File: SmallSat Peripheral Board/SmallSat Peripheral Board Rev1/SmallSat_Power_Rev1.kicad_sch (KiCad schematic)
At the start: 23 parts

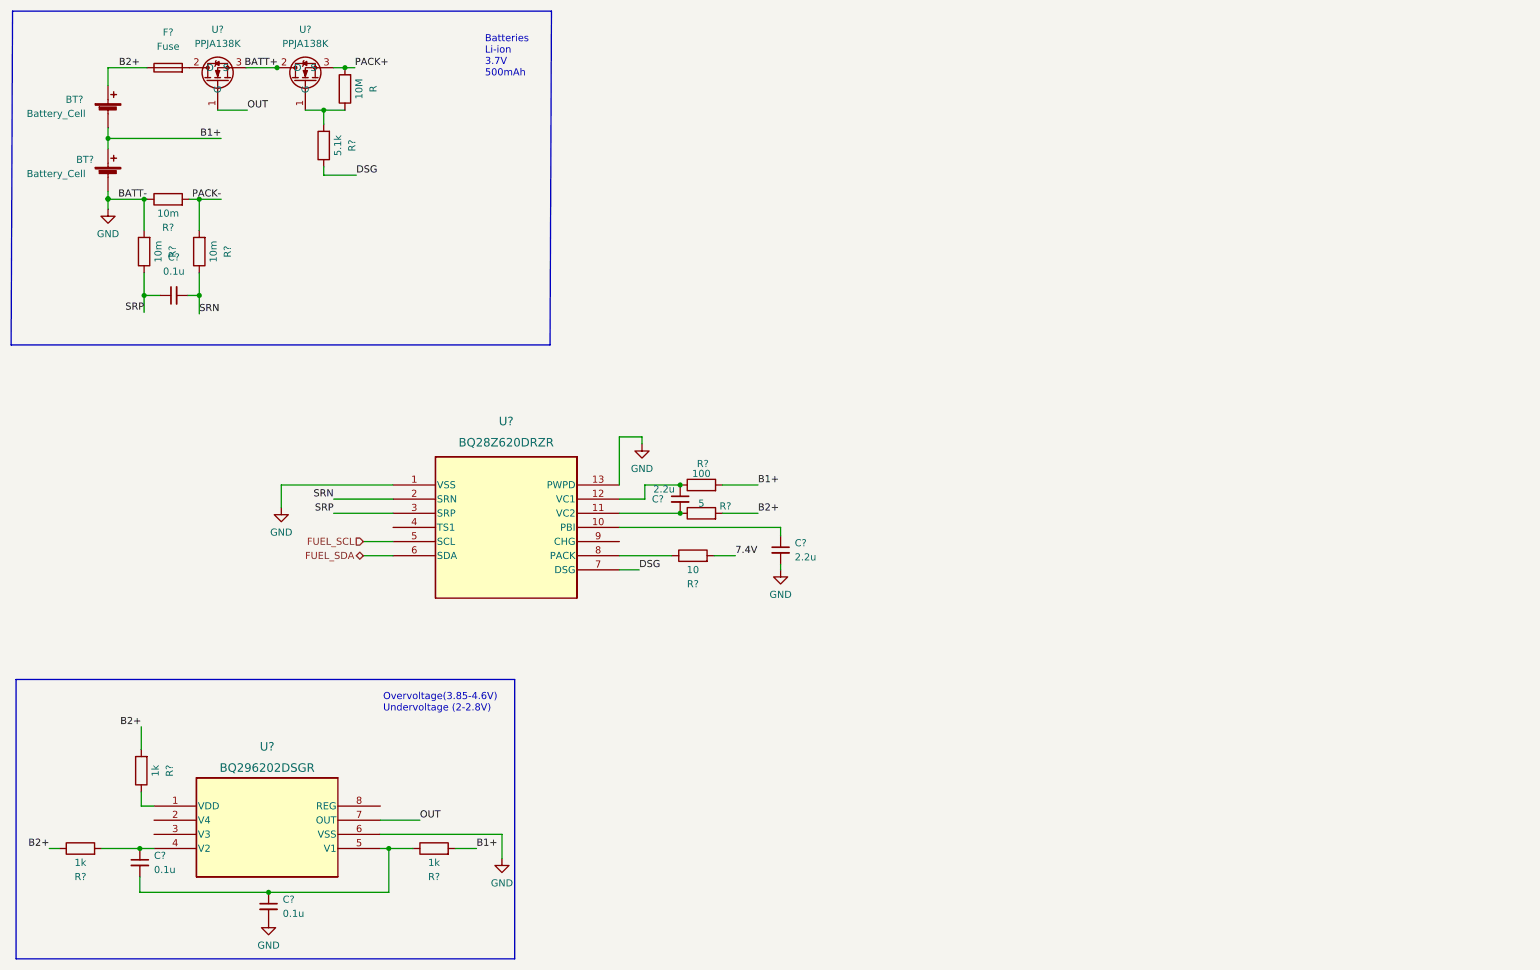
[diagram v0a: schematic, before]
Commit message: Finished First Try for Power Board
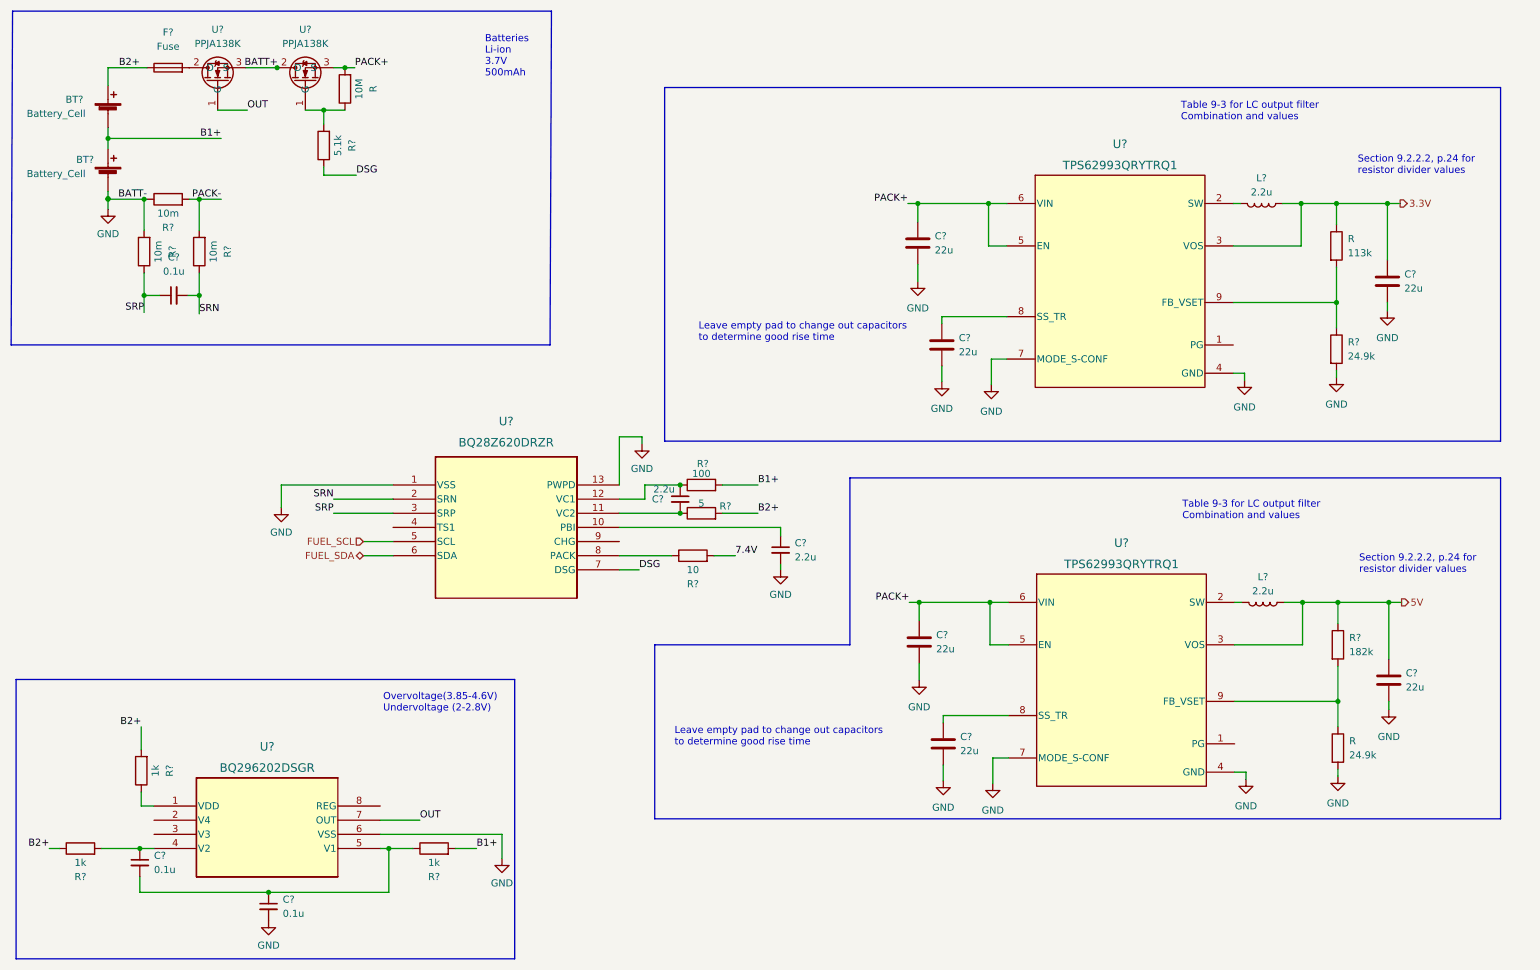
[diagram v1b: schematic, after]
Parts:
- added C? (x6): 22u, symbol Device:C
- added L? (x2): 2.2u, symbol Device:L
- added R, R?: 24.9k, symbol Device:R
- added R: 113k, symbol Device:R
- added R?: 182k, symbol Device:R
- added U? (x2): TPS62993QRYTRQ1, RYT0009A-MFG, symbol SmallSat-Peripherals-Board:TPS62993QRYTRQ1
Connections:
- net GND: now also C?.2, C?.2, C?.2, C?.2, C?.2, C?.2, R.2, R?.2, U?.4 (GND), U?.4 (GND), U?.7 (MODE_S-CONF), U?.7 (MODE_S-CONF)
- net PACK+: now also C?.1, C?.1, U?.5 (EN), U?.5 (EN), U?.6 (VIN), U?.6 (VIN)
- new net: C?.1, U?.8 (SS_TR) (x2)
- new net: L?.2, U?.2 (SW) (x2)
- new net: R.1, R?.2, U?.9 (FB_VSET)
- new net: R.2, R?.1, U?.9 (FB_VSET)
- new net 3.3V: C?.1, L?.1, R.1, U?.3 (VOS)
- new net 5V: C?.1, L?.1, R?.1, U?.3 (VOS)
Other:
- note added: "Leave empty pad to change out capacitors to determine good rise time"
- note added: "Section 9.2.2.2, p.24 for resistor divider values"
- note added: "Table 9-3 for LC output filter Combination and values"

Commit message: PB-order version
Sent the order in for Rev 1 power board with this version
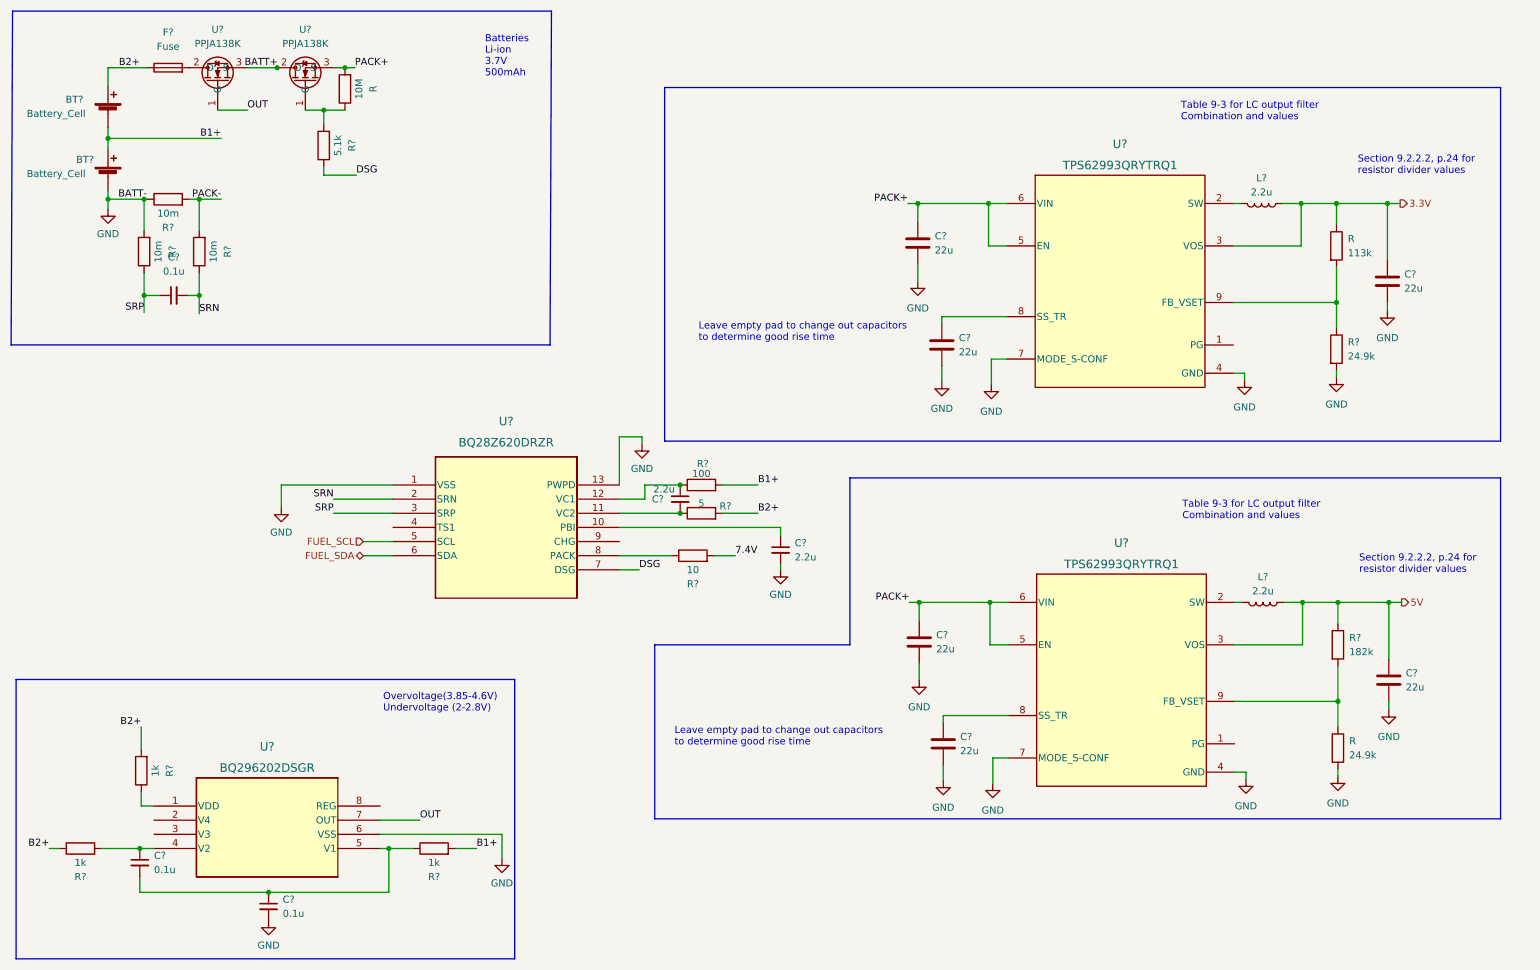
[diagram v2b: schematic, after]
